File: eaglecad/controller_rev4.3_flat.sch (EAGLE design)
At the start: 134 parts, among them J2 J-SAMTEC-TFM-120-X1-XXX-D-RA, U100 STM32L452XX_QFPN48, U101 TCAN330, U200 TPS63070, U300 STSPIN230, U301 TSV991ILT, U302 AS5047P, U400 STSPIN250, U401 TSV991ILT, X101 ABM10-16MHz

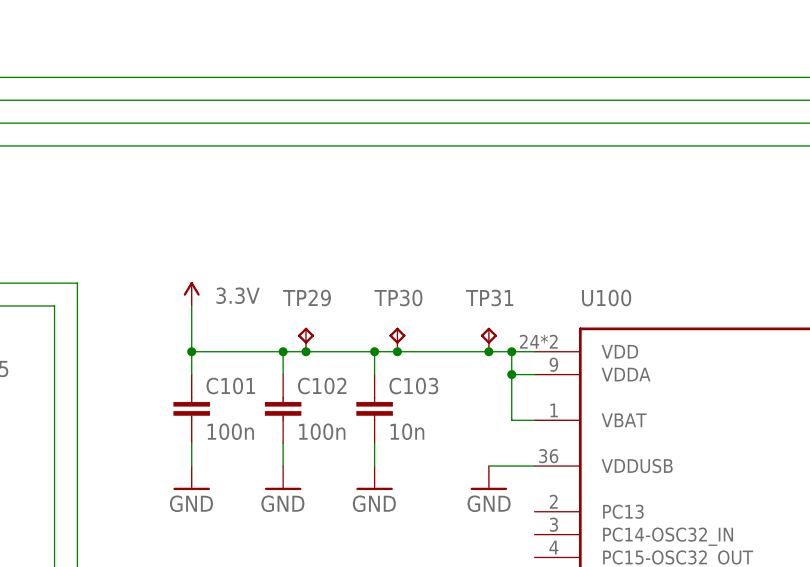
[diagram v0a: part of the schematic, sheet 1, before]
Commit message: Flat ready for review for real this time
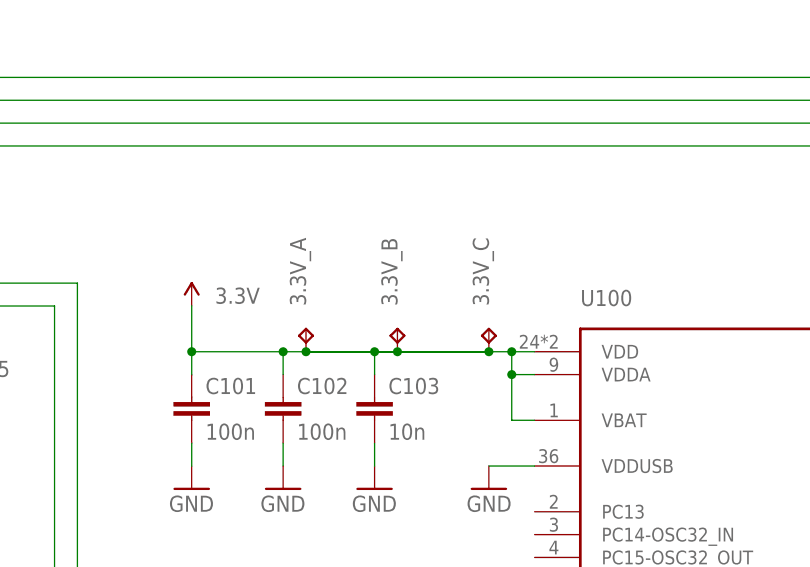
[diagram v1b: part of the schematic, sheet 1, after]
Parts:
- renumbered TP29 to 3.3V_A, TP30 to 3.3V_B, TP31 to 3.3V_C
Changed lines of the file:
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@@
 <part name="CAN_SIL" library="oresat-misc" deviceset="TEST-POINT-LARGE" device=""/>
 <part name="CAN_RX" library="oresat-misc" deviceset="TEST-POINT-LARGE" device=""/>
-<part name="TP29" library="oresat-misc" deviceset="TEST-POINT-LARGE" device=""/>
-<part name="TP30" library="oresat-misc" deviceset="TEST-POINT-LARGE" device=""/>
-<part name="TP31" library="oresat-misc" deviceset="TEST-POINT-LARGE" device=""/>
+<part name="3.3V_C" library="oresat-misc" deviceset="TEST-POINT-LARGE" device=""/>
+<part name="3.3V_A" library="oresat-misc" deviceset="TEST-POINT-LARGE" device=""/>
+<part name="3.3V_B" library="oresat-misc" deviceset="TEST-POINT-LARGE" device=""/>
 <part name="SWD1" library="J-CNC-3220-10-0100-00-ARM-SWD-port" deviceset="1.27MM-SWD-CONNECTOR" device=""/>
 <part name="J1" library="SparkFun-Connectors" library_urn="urn:adsk.eagle:library:513" deviceset="6_PIN_SERIAL_TARGET" device="SILK" package3d_urn="urn:adsk.eagle:package:37995/1"/>
@@
 <attribute name="NAME" x="246.38" y="53.34" size="1.778" layer="95"/>
 </instance>
-<instance part="TP29" gate="G$1" x="251.46" y="137.16" smashed="yes">
-<attribute name="NAME" x="248.92" y="139.7" size="1.778" layer="95"/>
-</instance>
-<instance part="TP30" gate="G$1" x="261.62" y="137.16" smashed="yes">
-<attribute name="NAME" x="259.08" y="139.7" size="1.778" layer="95"/>
-</instance>
-<instance part="TP31" gate="G$1" x="271.78" y="137.16" smashed="yes">
-<attribute name="NAME" x="269.24" y="139.7" size="1.778" layer="95"/>
+<instance part="3.3V_C" gate="G$1" x="271.78" y="137.16" smashed="yes">
+<attribute name="NAME" x="271.78" y="139.7" size="1.778" layer="95" rot="R90"/>
+</instance>
+<instance part="3.3V_A" gate="G$1" x="251.46" y="137.16" smashed="yes">
+<attribute name="NAME" x="251.46" y="139.7" size="1.778" layer="95" rot="R90"/>
+</instance>
+<instance part="3.3V_B" gate="G$1" x="261.62" y="137.16" smashed="yes">
+<attribute name="NAME" x="261.62" y="139.7" size="1.778" layer="95" rot="R90"/>
 </instance>
 <instance part="SWD1" gate="J" x="119.38" y="83.82" smashed="yes" rot="MR0">
@@
 <wire x1="274.32" y1="127" x2="274.32" y2="132.08" width="0.1524" layer="91"/>
 <junction x="274.32" y="132.08"/>
-<wire x1="274.32" y1="134.62" x2="271.78" y2="134.62" width="0.1524" layer="91"/>
+<wire x1="274.32" y1="134.62" x2="261.62" y2="134.62" width="0.1524" layer="91"/>
 <pinref part="SUPPLY6" gate="G$1" pin="3.3V"/>
-<wire x1="271.78" y1="134.62" x2="261.62" y2="134.62" width="0.1524" layer="91"/>
-<wire x1="261.62" y1="134.62" x2="259.08" y2="134.62" width="0.1524" layer="91"/>
-<wire x1="259.08" y1="134.62" x2="251.46" y2="134.62" width="0.1524" layer="91"/>
-<wire x1="251.46" y1="134.62" x2="248.92" y2="134.62" width="0.1524" layer="91"/>
+<wire x1="261.62" y1="134.62" x2="251.46" y2="134.62" width="0.1524" layer="91"/>
+<wire x1="251.46" y1="134.62" x2="259.08" y2="134.62" width="0.1524" layer="91"/>
+<wire x1="259.08" y1="134.62" x2="271.78" y2="134.62" width="0.1524" layer="91"/>
+<wire x1="271.78" y1="134.62" x2="248.92" y2="134.62" width="0.1524" layer="91"/>
 <wire x1="248.92" y1="134.62" x2="238.76" y2="134.62" width="0.1524" layer="91"/>
 <wire x1="238.76" y1="139.7" x2="238.76" y2="134.62" width="0.1524" layer="91"/>
@@
 <wire x1="259.08" y1="132.08" x2="259.08" y2="134.62" width="0.1524" layer="91"/>
 <junction x="259.08" y="134.62"/>
-<pinref part="TP29" gate="G$1" pin="TP"/>
+<pinref part="3.3V_C" gate="G$1" pin="TP"/>
+<junction x="271.78" y="134.62"/>
+<pinref part="3.3V_A" gate="G$1" pin="TP"/>
 <junction x="251.46" y="134.62"/>
-<pinref part="TP30" gate="G$1" pin="TP"/>
+<pinref part="3.3V_B" gate="G$1" pin="TP"/>
 <junction x="261.62" y="134.62"/>
-<pinref part="TP31" gate="G$1" pin="TP"/>
-<junction x="271.78" y="134.62"/>
-</segment>
-<segment>
+</segment>
+<segment>
